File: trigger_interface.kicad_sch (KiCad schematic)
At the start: 27 parts, among them J10 Conn_Coaxial_Small, J11 Conn_Coaxial_Small, J12 Conn_Coaxial_Small, J3 RJHSE508002, J4 Conn_Coaxial_Small, J5 Conn_Coaxial_Small, J6 Conn_Coaxial_Small, J7 Conn_Coaxial_Small, J9 Conn_Coaxial_Small, U10 SN65MLVD206BD, U11 SN65MLVD206BD, U12 SN65MLVD206BD, U13 SN65LVDT348D, U9 SN65MLVD206BD

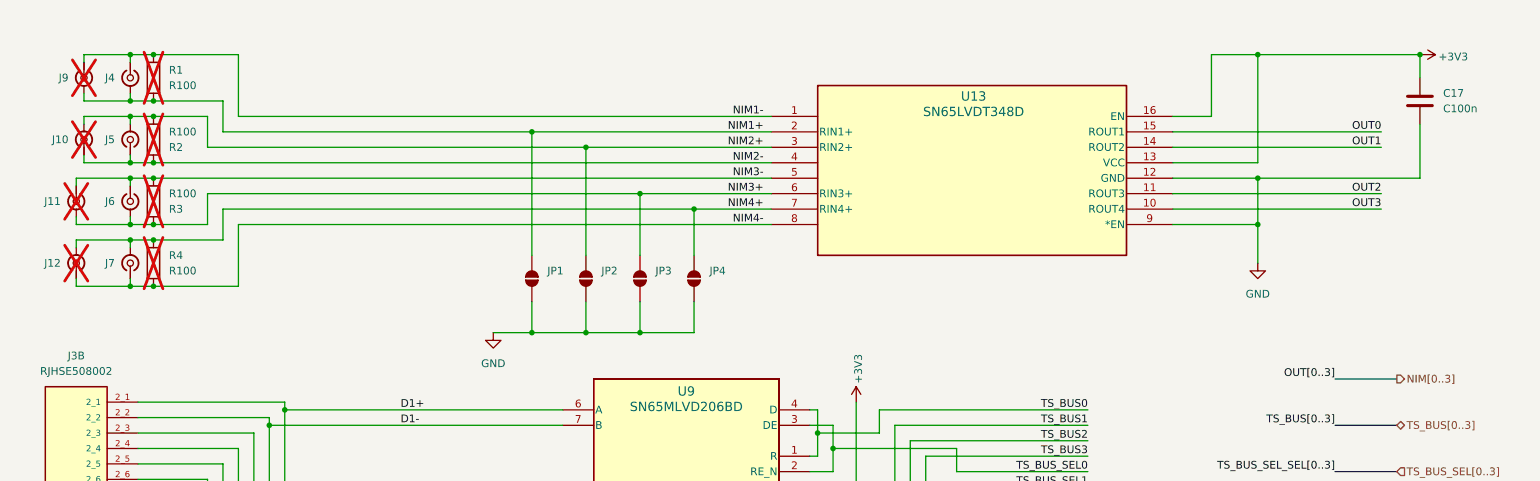
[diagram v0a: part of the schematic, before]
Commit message: v2
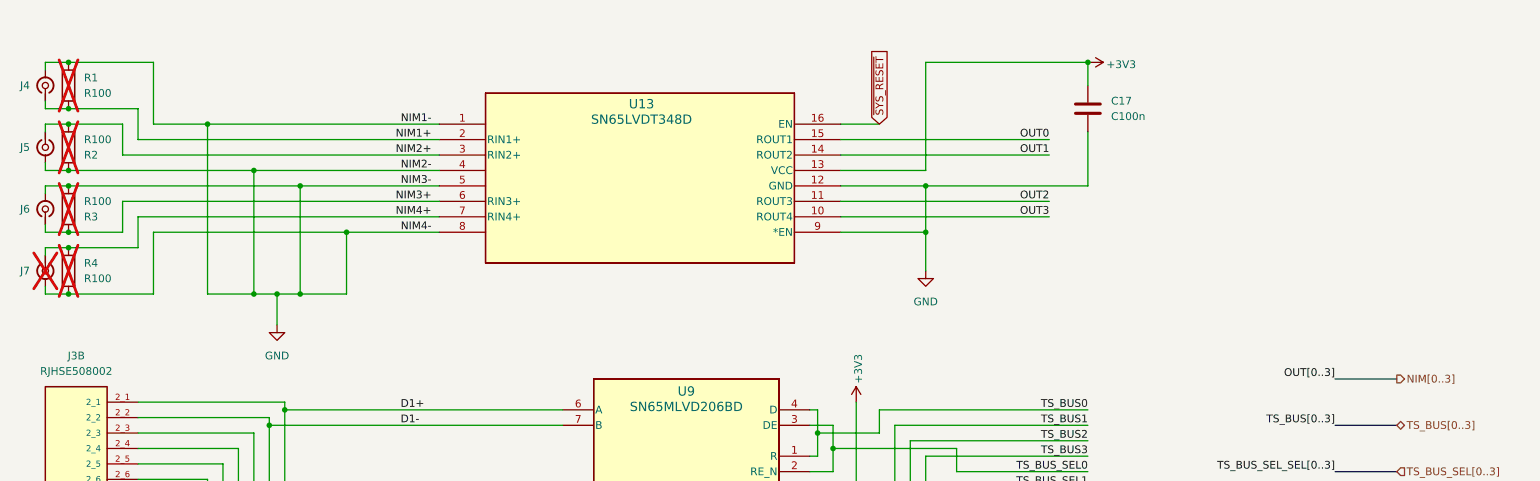
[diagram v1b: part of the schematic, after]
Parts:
- removed J10, J11, J12, J9: Conn_Coaxial_Small, Connector_Coaxial:SMA_Amphenol_901-143_Horizontal, symbol Connector:Conn_Coaxial_Small
- removed JP1, JP2, JP3, JP4: SolderJumper_2_Open, Jumper:SolderJumper-2_P1.3mm_Open_RoundedPad1.0x1.5mm, symbol Jumper:SolderJumper_2_Open
- J7: now not fitted
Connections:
- net +3V3: no longer U13.16 (EN)
- net GND: now also J4.2 (Ext), J5.2 (Ext), J6.2 (Ext), J7.2 (Ext), R1.1, R2.1, R3.2, R4.2, U13.1, U13.4, U13.5, U13.8
- net NIM1+: now also J4.1 (In); no longer J4.2 (Ext)
- net NIM2+: now also J5.1 (In); no longer J5.2 (Ext)
- net NIM3+: now also J6.1 (In); no longer J6.2 (Ext)
- net NIM4+: now also J7.1 (In); no longer J7.2 (Ext)
- removed net NIM1-: J4.1 (In), R1.1, U13.1
- removed net NIM2-: J5.1 (In), R2.1, U13.4
- removed net NIM3-: J6.1 (In), R3.2, U13.5
- removed net NIM4-: J7.1 (In), R4.2, U13.8
- new net ~{SYS_RESET}: U13.16 (EN)
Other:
- company: (none) -> MIT SpinQuest DAQ Group
- title: (none) -> BeagleV Fire TDC Cape
- moved on the sheet: C17, J4, J5, J6, R1, R2, R3, R4, U13
